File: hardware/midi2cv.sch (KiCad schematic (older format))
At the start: 2 parts

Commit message: First preliminary board design
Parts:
- removed J?: Conn_02x10_Odd_Even, Connector_PinSocket_2.00mm:PinSocket_2x10_P2.00mm_Vertical, symbol Connector_Generic:Conn_02x10_Odd_Even
- removed J?: Conn_02x10_Odd_Even, Connector_PinHeader_2.00mm:PinHeader_2x10_P2.00mm_Vertical, symbol Connector_Generic:Conn_02x10_Odd_Even
- added J1, J2: Conn_02x06_Odd_Even, Connector_PinSocket_2.54mm:PinSocket_2x06_P2.54mm_Vertical, symbol Connector_Generic:Conn_02x06_Odd_Even
- added J3: Conn_02x10_Odd_Even, Connector_PinSocket_2.54mm:PinSocket_2x12_P2.54mm_Vertical, symbol Connector_Generic:Conn_02x12_Odd_Even
- added J4, J5: Conn_02x06_Odd_Even, Connector_PinHeader_2.54mm:PinHeader_2x06_P2.54mm_Vertical, symbol Connector_Generic:Conn_02x06_Odd_Even
- added J6: Conn_02x10_Odd_Even, Connector_PinHeader_2.54mm:PinHeader_2x12_P2.54mm_Vertical, symbol Connector_Generic:Conn_02x12_Odd_Even
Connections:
- net labels added: +3.3V, 1_16_out_back, 1_16_out_front, GND, button_a_back, button_a_front, button_b_back, button_b_front, button_c_back, button_c_front, button_d_back, button_d_front, clock_out_back, clock_out_front, cv_in_a_back, cv_in_a_front, cv_in_b_back, cv_in_b_front, dac4_out_a_back, dac4_out_a_front, dac4_out_b_back, dac4_out_b_front, dac4_out_c_back, dac4_out_c_front, dac4_out_d_back, dac4_out_d_front, dac8_out_a_back, dac8_out_a_front, dac8_out_b_back, dac8_out_b_front, dac8_out_c_back, dac8_out_c_front, dac8_out_d_back, dac8_out_d_front, dac8_out_e_back, dac8_out_e_front, dac8_out_f_back, dac8_out_f_front, dac8_out_g_back, dac8_out_g_front, dac8_out_h_back, dac8_out_h_front, gate_out_a_back, gate_out_a_front, gate_out_b_back, gate_out_b_front, gate_out_c_back, gate_out_c_front, gate_out_d_back, gate_out_d_front, jack_detect_back, jack_detect_front, led_out_a_b_back, led_out_a_b_front, led_out_a_g_back, led_out_a_g_front, led_out_a_r_back, led_out_a_r_front, led_out_b_b_back, led_out_b_b_front, led_out_b_g_back, led_out_b_g_front, led_out_b_r_back, led_out_b_r_front, led_out_c_b_back, led_out_c_b_front, led_out_c_g_back, led_out_c_g_front, led_out_c_r_back, led_out_c_r_front, led_out_d_b_back, led_out_d_b_front, led_out_d_g_back, led_out_d_g_front, led_out_d_r_back, led_out_d_r_front, midi_in+_back, midi_in+_front, midi_in-_back, midi_in-_front, run_out_back, run_out_front, var_out_back, var_out_front
- wire segments 0 -> 2
- no-connect marks 0 -> 4

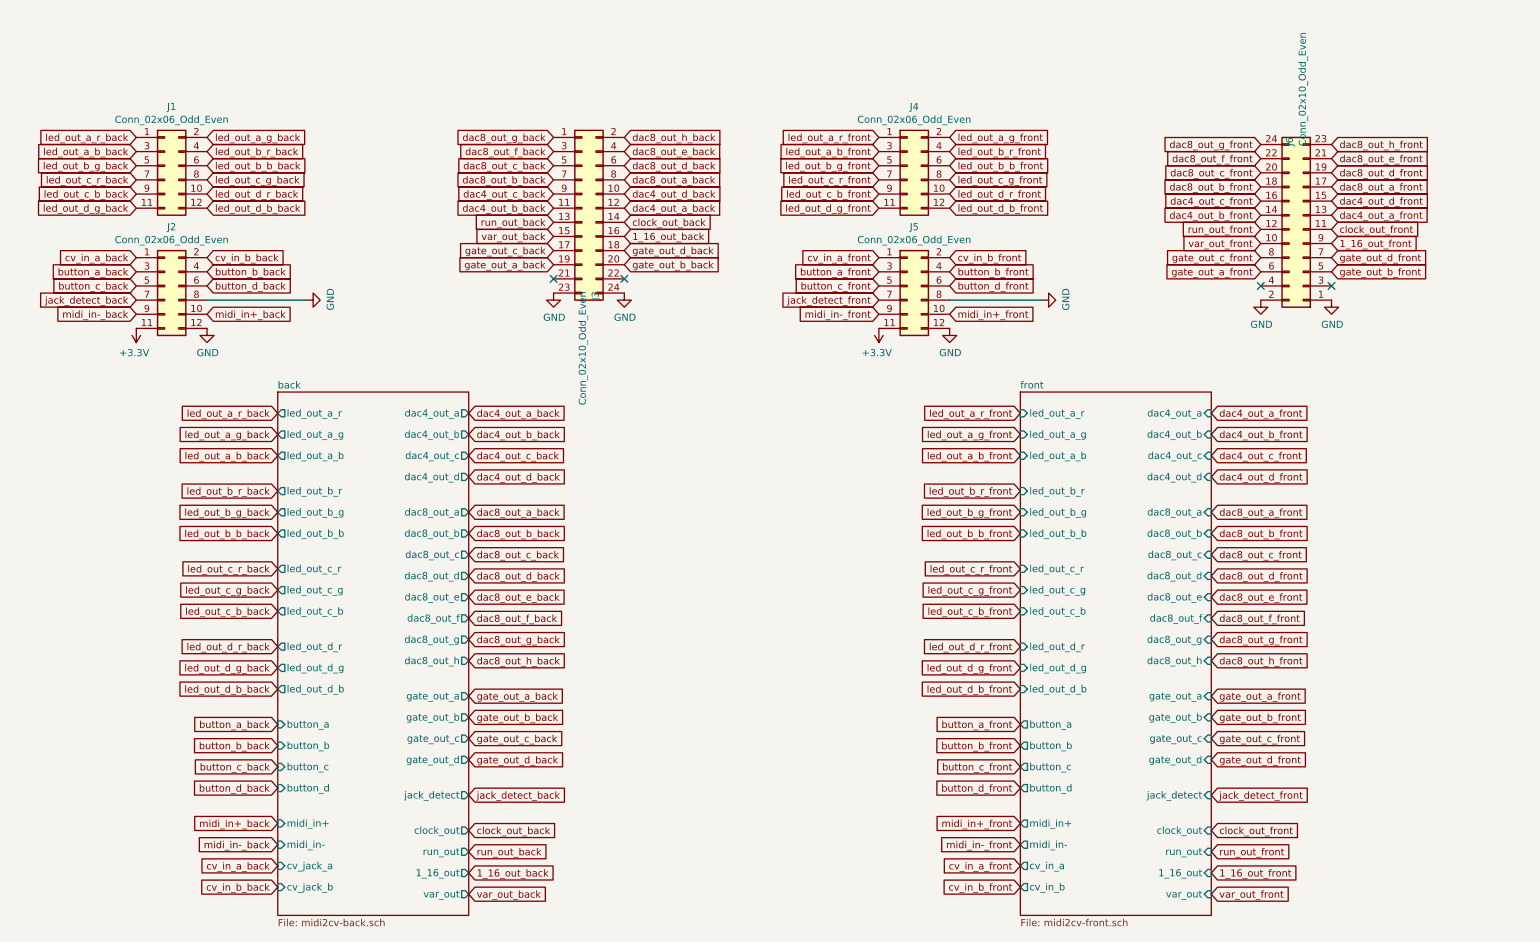
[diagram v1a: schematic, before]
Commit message: Layed out stretched design
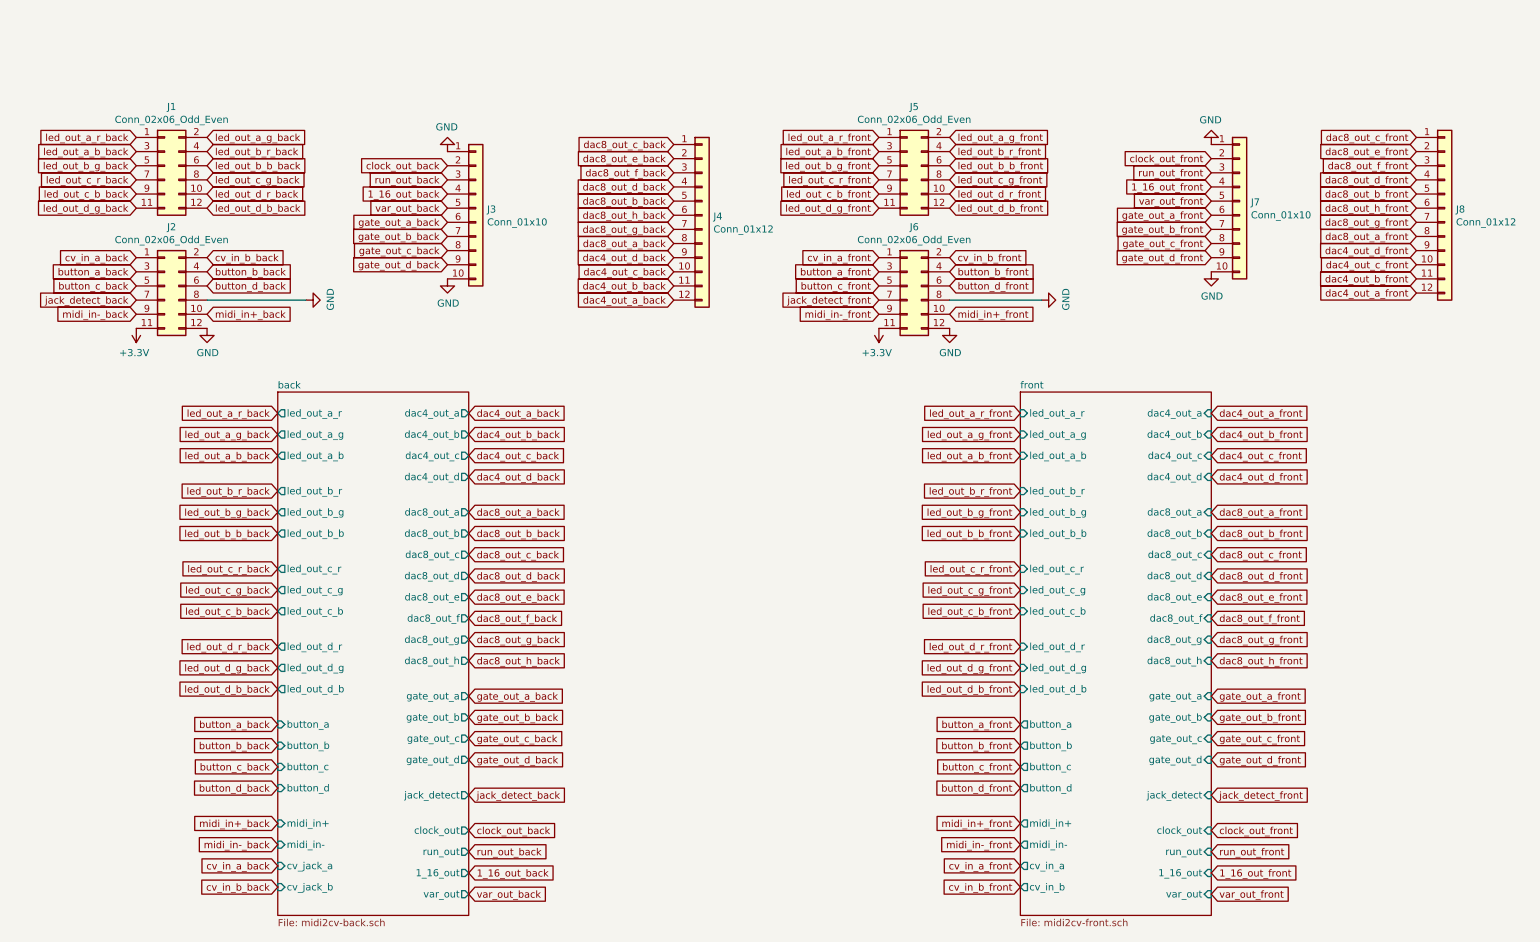
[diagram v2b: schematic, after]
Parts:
- removed J3: Conn_02x10_Odd_Even, Connector_PinSocket_2.54mm:PinSocket_2x12_P2.54mm_Vertical, symbol Connector_Generic:Conn_02x12_Odd_Even
- removed J6: Conn_02x10_Odd_Even, Connector_PinHeader_2.54mm:PinHeader_2x12_P2.54mm_Vertical, symbol Connector_Generic:Conn_02x12_Odd_Even
- added J3: Conn_01x10, Connector_PinSocket_2.54mm:PinSocket_1x10_P2.54mm_Vertical, symbol Connector_Generic:Conn_01x10
- added J4: Conn_01x12, Connector_PinSocket_2.54mm:PinSocket_1x12_P2.54mm_Vertical, symbol Connector_Generic:Conn_01x12
- added J7: Conn_01x10, Connector_PinHeader_2.54mm:PinHeader_1x10_P2.54mm_Vertical, symbol Connector_Generic:Conn_01x10
- added J8: Conn_01x12, Connector_PinHeader_2.54mm:PinHeader_1x12_P2.54mm_Vertical, symbol Connector_Generic:Conn_01x12
- renumbered J4 to J5, J5 to J6
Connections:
- net 1_16_out_back: now also J3.4 (Pin_4)
- net 1_16_out_front: now also J7.4 (Pin_4)
- net GND: now also J3.1 (Pin_1), J3.10 (Pin_10), J7.1 (Pin_1), J7.10 (Pin_10)
- net clock_out_back: now also J3.2 (Pin_2)
- net clock_out_front: now also J7.2 (Pin_2)
- net dac4_out_a_back: now also J4.12 (Pin_12)
- net dac4_out_a_front: now also J8.12 (Pin_12)
- net dac4_out_b_back: now also J4.11 (Pin_11)
- net dac4_out_b_front: now also J8.11 (Pin_11)
- net dac4_out_c_back: now also J4.10 (Pin_10)
- net dac4_out_c_front: now also J8.10 (Pin_10)
- net dac4_out_d_back: now also J4.9 (Pin_9)
- net dac4_out_d_front: now also J8.9 (Pin_9)
- net dac8_out_a_back: now also J4.8 (Pin_8)
- net dac8_out_a_front: now also J8.8 (Pin_8)
- net dac8_out_b_back: now also J4.5 (Pin_5)
- net dac8_out_b_front: now also J8.5 (Pin_5)
- net dac8_out_c_back: now also J4.1 (Pin_1)
- net dac8_out_c_front: now also J8.1 (Pin_1)
- net dac8_out_d_back: now also J4.4 (Pin_4)
- net dac8_out_d_front: now also J8.4 (Pin_4)
- net dac8_out_e_back: now also J4.2 (Pin_2)
- net dac8_out_e_front: now also J8.2 (Pin_2)
- net dac8_out_f_back: now also J4.3 (Pin_3)
- net dac8_out_f_front: now also J8.3 (Pin_3)
- net dac8_out_g_back: now also J4.7 (Pin_7)
- net dac8_out_g_front: now also J8.7 (Pin_7)
- net dac8_out_h_back: now also J4.6 (Pin_6)
- net dac8_out_h_front: now also J8.6 (Pin_6)
- net gate_out_a_back: now also J3.6 (Pin_6)
- net gate_out_a_front: now also J7.6 (Pin_6)
- net gate_out_b_back: now also J3.7 (Pin_7)
- net gate_out_b_front: now also J7.7 (Pin_7)
- net gate_out_c_back: now also J3.8 (Pin_8)
- net gate_out_c_front: now also J7.8 (Pin_8)
- net gate_out_d_back: now also J3.9 (Pin_9)
- net gate_out_d_front: now also J7.9 (Pin_9)
- net run_out_back: now also J3.3 (Pin_3)
- net run_out_front: now also J7.3 (Pin_3)
- net var_out_back: now also J3.5 (Pin_5)
- net var_out_front: now also J7.5 (Pin_5)
- no-connect marks 4 -> 0

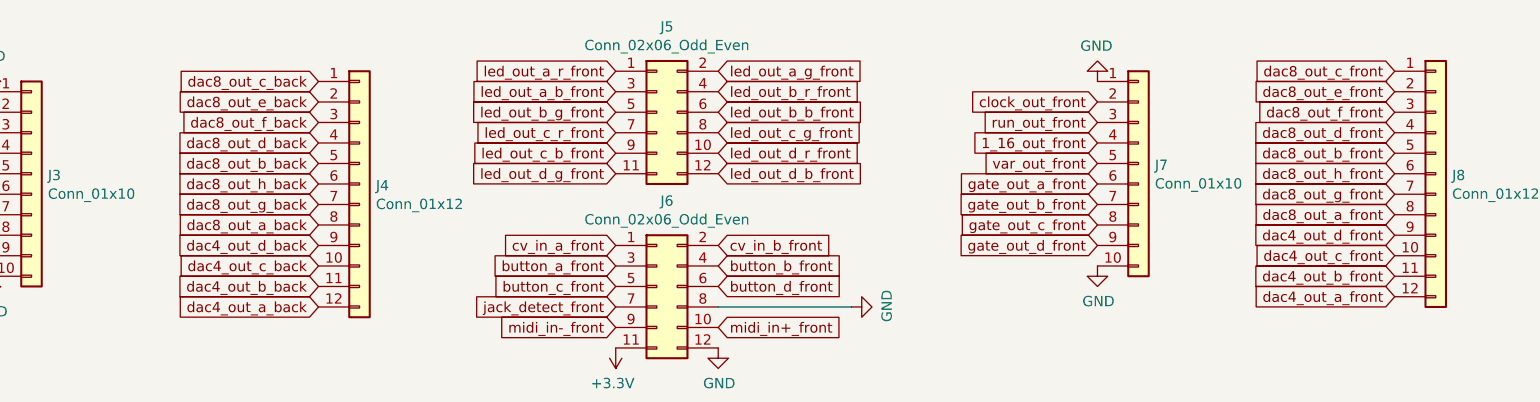
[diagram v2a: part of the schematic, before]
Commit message: wire up ad5328
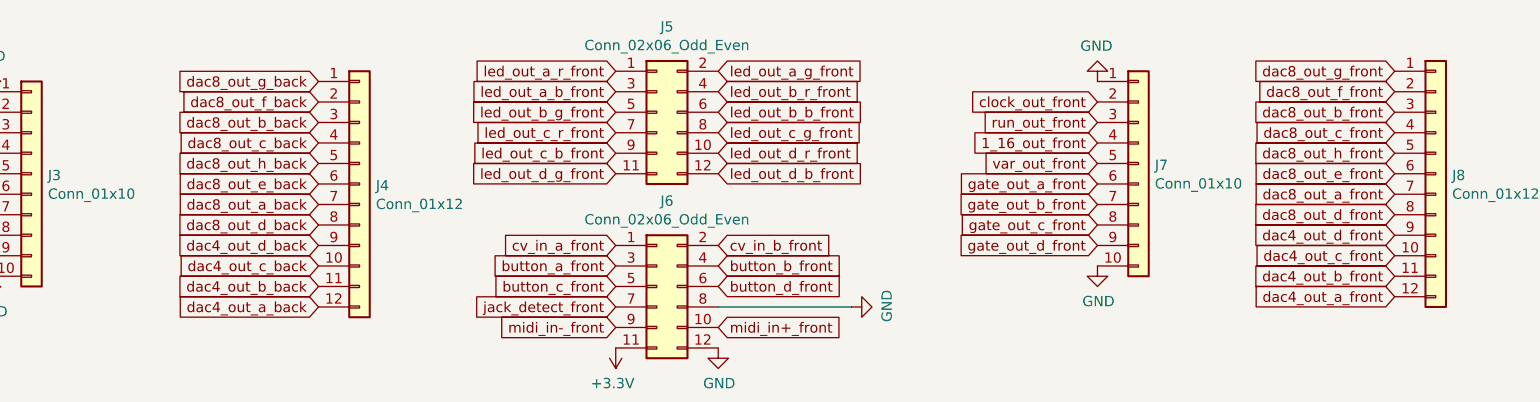
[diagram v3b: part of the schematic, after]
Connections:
- net dac8_out_a_back: now also J4.7 (Pin_7); no longer J4.8 (Pin_8)
- net dac8_out_a_front: now also J8.7 (Pin_7); no longer J8.8 (Pin_8)
- net dac8_out_b_back: now also J4.3 (Pin_3); no longer J4.5 (Pin_5)
- net dac8_out_b_front: now also J8.3 (Pin_3); no longer J8.5 (Pin_5)
- net dac8_out_c_back: now also J4.4 (Pin_4); no longer J4.1 (Pin_1)
- net dac8_out_c_front: now also J8.4 (Pin_4); no longer J8.1 (Pin_1)
- net dac8_out_d_back: now also J4.8 (Pin_8); no longer J4.4 (Pin_4)
- net dac8_out_d_front: now also J8.8 (Pin_8); no longer J8.4 (Pin_4)
- net dac8_out_e_back: now also J4.6 (Pin_6); no longer J4.2 (Pin_2)
- net dac8_out_e_front: now also J8.6 (Pin_6); no longer J8.2 (Pin_2)
- net dac8_out_f_back: now also J4.2 (Pin_2); no longer J4.3 (Pin_3)
- net dac8_out_f_front: now also J8.2 (Pin_2); no longer J8.3 (Pin_3)
- net dac8_out_g_back: now also J4.1 (Pin_1); no longer J4.7 (Pin_7)
- net dac8_out_g_front: now also J8.1 (Pin_1); no longer J8.7 (Pin_7)
- net dac8_out_h_back: now also J4.5 (Pin_5); no longer J4.6 (Pin_6)
- net dac8_out_h_front: now also J8.5 (Pin_5); no longer J8.6 (Pin_6)
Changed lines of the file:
@@
 Text GLabel 1650 1650 0    50   Input ~ 0
 cv_in_a_back
-Text GLabel 5450 1950 0    50   Input ~ 0
-dac4_out_a_back
-Text GLabel 5450 1750 0    50   Input ~ 0
-dac4_out_c_back
-Text GLabel 5450 1550 0    50   Input ~ 0
-dac8_out_a_back
-Text GLabel 5450 850  0    50   Input ~ 0
-dac8_out_c_back
-Text GLabel 5450 950  0    50   Input ~ 0
-dac8_out_e_back
-Text GLabel 5450 1450 0    50   Input ~ 0
-dac8_out_g_back
 Text GLabel 3850 1400 0    50   Input ~ 0
 gate_out_a_back
@@
 	-1   0    0    1
 $EndComp
-Text GLabel 5450 1850 0    50   Input ~ 0
-dac4_out_b_back
-Text GLabel 5450 1650 0    50   Input ~ 0
-dac4_out_d_back
-Text GLabel 5450 1250 0    50   Input ~ 0
-dac8_out_b_back
-Text GLabel 5450 1150 0    50   Input ~ 0
-dac8_out_d_back
-Text GLabel 5450 1050 0    50   Input ~ 0
-dac8_out_f_back
-Text GLabel 5450 1350 0    50   Input ~ 0
-dac8_out_h_back
 Text GLabel 3850 1500 0    50   Input ~ 0
 gate_out_b_back
@@
 Text GLabel 10700 1900 0    50   Input ~ 0
 dac4_out_a_front
-Text GLabel 10700 1500 0    50   Input ~ 0
+Text GLabel 10700 1400 0    50   Input ~ 0
 dac8_out_a_front
-Text GLabel 10700 900  0    50   Input ~ 0
+Text GLabel 10700 1300 0    50   Input ~ 0
 dac8_out_e_front
 Text GLabel 6900 1950 0    50   Input ~ 0
@@
 Text GLabel 10700 1600 0    50   Input ~ 0
 dac4_out_d_front
-Text GLabel 10700 1100 0    50   Input ~ 0
+Text GLabel 10700 1500 0    50   Input ~ 0
 dac8_out_d_front
-Text GLabel 10700 1300 0    50   Input ~ 0
+Text GLabel 10700 1200 0    50   Input ~ 0
 dac8_out_h_front
 Text GLabel 9250 1450 0    50   Input ~ 0
@@
 	1    0    0    -1
 $EndComp
+Text GLabel 10700 900  0    50   Input ~ 0
+dac8_out_f_front
 Text GLabel 10700 1000 0    50   Input ~ 0
-dac8_out_f_front
-Text GLabel 10700 1200 0    50   Input ~ 0
 dac8_out_b_front
 Text GLabel 10700 1800 0    50   Input ~ 0
@@
 Text GLabel 9250 1350 0    50   Input ~ 0
 gate_out_a_front
-Text GLabel 10700 1400 0    50   Input ~ 0
+Text GLabel 10700 800  0    50   Input ~ 0
 dac8_out_g_front
-Text GLabel 10700 800  0    50   Input ~ 0
+Text GLabel 10700 1100 0    50   Input ~ 0
 dac8_out_c_front
 Text GLabel 10700 1700 0    50   Input ~ 0
 dac4_out_c_front
+Text GLabel 5450 1250 0    50   Input ~ 0
+dac8_out_h_back
+Text GLabel 5450 950  0    50   Input ~ 0
+dac8_out_f_back
+Text GLabel 5450 1550 0    50   Input ~ 0
+dac8_out_d_back
+Text GLabel 5450 1050 0    50   Input ~ 0
+dac8_out_b_back
+Text GLabel 5450 1850 0    50   Input ~ 0
+dac4_out_b_back
+Text GLabel 5450 850  0    50   Input ~ 0
+dac8_out_g_back
+Text GLabel 5450 1350 0    50   Input ~ 0
+dac8_out_e_back
+Text GLabel 5450 1150 0    50   Input ~ 0
+dac8_out_c_back
+Text GLabel 5450 1450 0    50   Input ~ 0
+dac8_out_a_back
+Text GLabel 5450 1750 0    50   Input ~ 0
+dac4_out_c_back
+Text GLabel 5450 1650 0    50   Input ~ 0
+dac4_out_d_back
+Text GLabel 5450 1950 0    50   Input ~ 0
+dac4_out_a_back
 $EndSCHEMATC

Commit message: make back compatible with old front
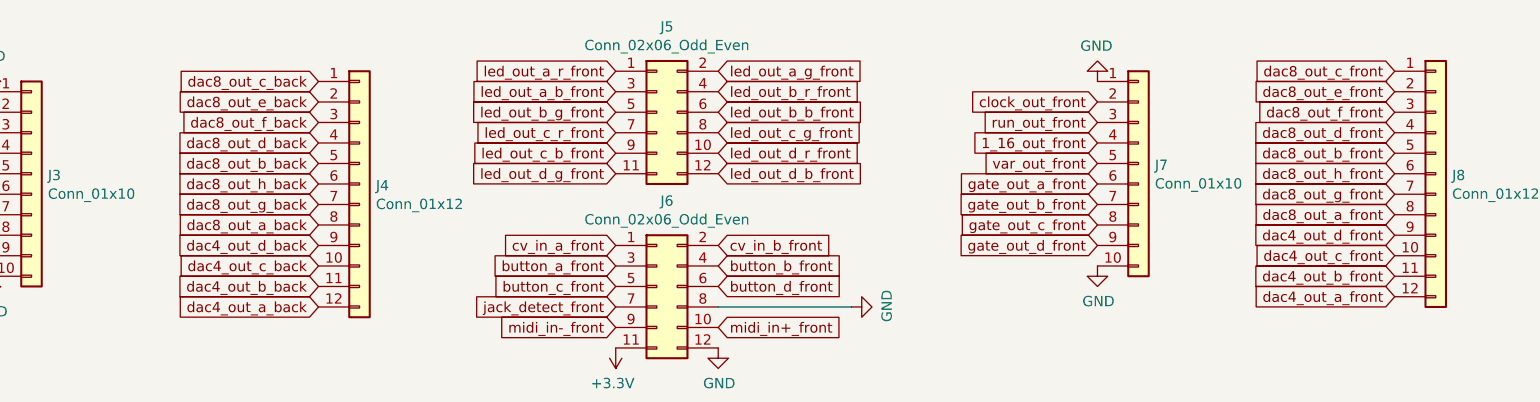
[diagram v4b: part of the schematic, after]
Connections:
- net dac8_out_a_back: now also J4.8 (Pin_8); no longer J4.7 (Pin_7)
- net dac8_out_a_front: now also J8.8 (Pin_8); no longer J8.7 (Pin_7)
- net dac8_out_b_back: now also J4.5 (Pin_5); no longer J4.3 (Pin_3)
- net dac8_out_b_front: now also J8.5 (Pin_5); no longer J8.3 (Pin_3)
- net dac8_out_c_back: now also J4.1 (Pin_1); no longer J4.4 (Pin_4)
- net dac8_out_c_front: now also J8.1 (Pin_1); no longer J8.4 (Pin_4)
- net dac8_out_d_back: now also J4.4 (Pin_4); no longer J4.8 (Pin_8)
- net dac8_out_d_front: now also J8.4 (Pin_4); no longer J8.8 (Pin_8)
- net dac8_out_e_back: now also J4.2 (Pin_2); no longer J4.6 (Pin_6)
- net dac8_out_e_front: now also J8.2 (Pin_2); no longer J8.6 (Pin_6)
- net dac8_out_f_back: now also J4.3 (Pin_3); no longer J4.2 (Pin_2)
- net dac8_out_f_front: now also J8.3 (Pin_3); no longer J8.2 (Pin_2)
- net dac8_out_g_back: now also J4.7 (Pin_7); no longer J4.1 (Pin_1)
- net dac8_out_g_front: now also J8.7 (Pin_7); no longer J8.1 (Pin_1)
- net dac8_out_h_back: now also J4.6 (Pin_6); no longer J4.5 (Pin_5)
- net dac8_out_h_front: now also J8.6 (Pin_6); no longer J8.5 (Pin_5)
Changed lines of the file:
@@
 Text GLabel 10700 1900 0    50   Input ~ 0
 dac4_out_a_front
-Text GLabel 10700 1400 0    50   Input ~ 0
+Text GLabel 10700 1500 0    50   Input ~ 0
 dac8_out_a_front
-Text GLabel 10700 1300 0    50   Input ~ 0
+Text GLabel 10700 900  0    50   Input ~ 0
 dac8_out_e_front
 Text GLabel 6900 1950 0    50   Input ~ 0
@@
 Text GLabel 10700 1600 0    50   Input ~ 0
 dac4_out_d_front
-Text GLabel 10700 1500 0    50   Input ~ 0
+Text GLabel 10700 1100 0    50   Input ~ 0
 dac8_out_d_front
-Text GLabel 10700 1200 0    50   Input ~ 0
+Text GLabel 10700 1300 0    50   Input ~ 0
 dac8_out_h_front
 Text GLabel 9250 1450 0    50   Input ~ 0
@@
 	1    0    0    -1
 $EndComp
-Text GLabel 10700 900  0    50   Input ~ 0
+Text GLabel 10700 1000 0    50   Input ~ 0
 dac8_out_f_front
-Text GLabel 10700 1000 0    50   Input ~ 0
+Text GLabel 10700 1200 0    50   Input ~ 0
 dac8_out_b_front
 Text GLabel 10700 1800 0    50   Input ~ 0
@@
 Text GLabel 9250 1350 0    50   Input ~ 0
 gate_out_a_front
+Text GLabel 10700 1400 0    50   Input ~ 0
+dac8_out_g_front
 Text GLabel 10700 800  0    50   Input ~ 0
-dac8_out_g_front
-Text GLabel 10700 1100 0    50   Input ~ 0
 dac8_out_c_front
 Text GLabel 10700 1700 0    50   Input ~ 0
 dac4_out_c_front
+Text GLabel 5450 1350 0    50   Input ~ 0
+dac8_out_h_back
+Text GLabel 5450 1050 0    50   Input ~ 0
+dac8_out_f_back
+Text GLabel 5450 1150 0    50   Input ~ 0
+dac8_out_d_back
 Text GLabel 5450 1250 0    50   Input ~ 0
-dac8_out_h_back
-Text GLabel 5450 950  0    50   Input ~ 0
-dac8_out_f_back
-Text GLabel 5450 1550 0    50   Input ~ 0
-dac8_out_d_back
-Text GLabel 5450 1050 0    50   Input ~ 0
 dac8_out_b_back
 Text GLabel 5450 1850 0    50   Input ~ 0
 dac4_out_b_back
+Text GLabel 5450 1450 0    50   Input ~ 0
+dac8_out_g_back
+Text GLabel 5450 950  0    50   Input ~ 0
+dac8_out_e_back
 Text GLabel 5450 850  0    50   Input ~ 0
-dac8_out_g_back
-Text GLabel 5450 1350 0    50   Input ~ 0
-dac8_out_e_back
-Text GLabel 5450 1150 0    50   Input ~ 0
 dac8_out_c_back
-Text GLabel 5450 1450 0    50   Input ~ 0
+Text GLabel 5450 1550 0    50   Input ~ 0
 dac8_out_a_back
 Text GLabel 5450 1750 0    50   Input ~ 0
